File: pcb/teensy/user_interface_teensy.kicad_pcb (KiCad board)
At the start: 2 copper layers, 63.5 x 40.6 mm, 15 parts, among them P1 HEADER_02X08_SMD, SW1 SPST_SLIDE_AS, U1 TLE7230R

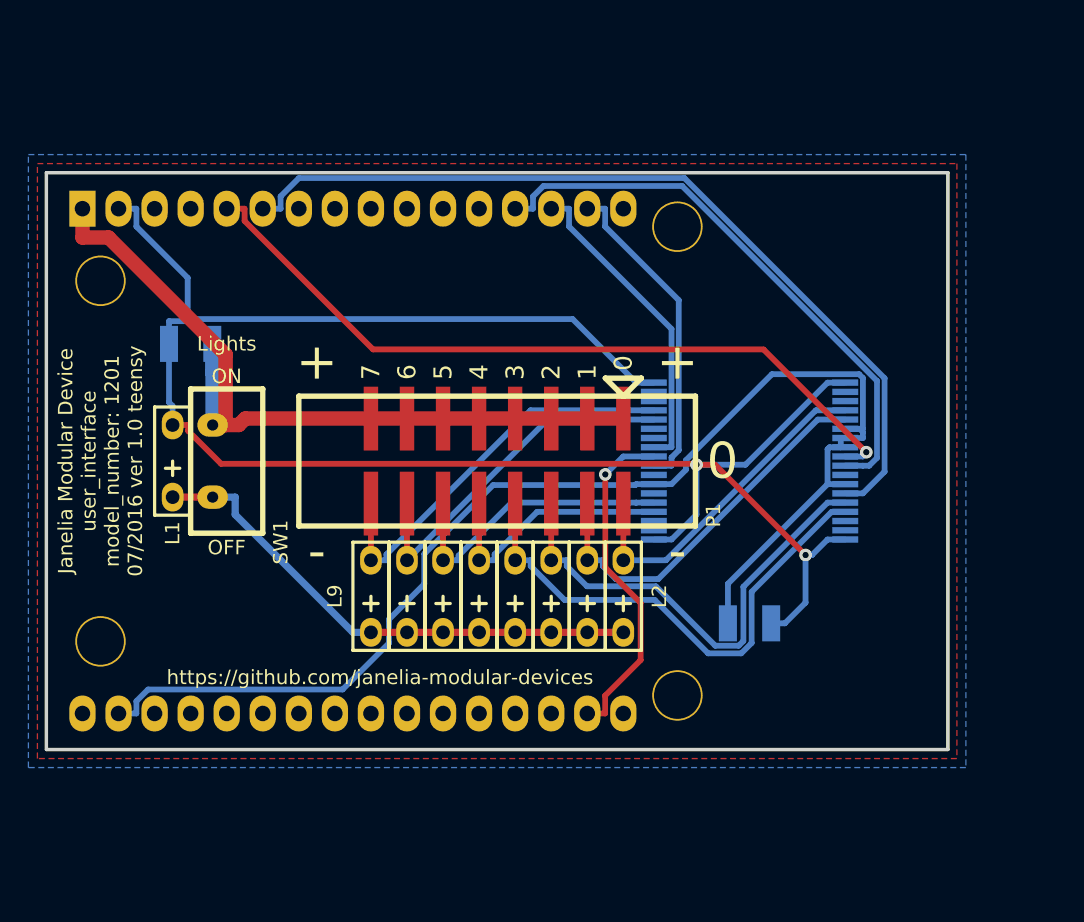
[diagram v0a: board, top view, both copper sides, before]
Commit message: Finished pcb v1.0.
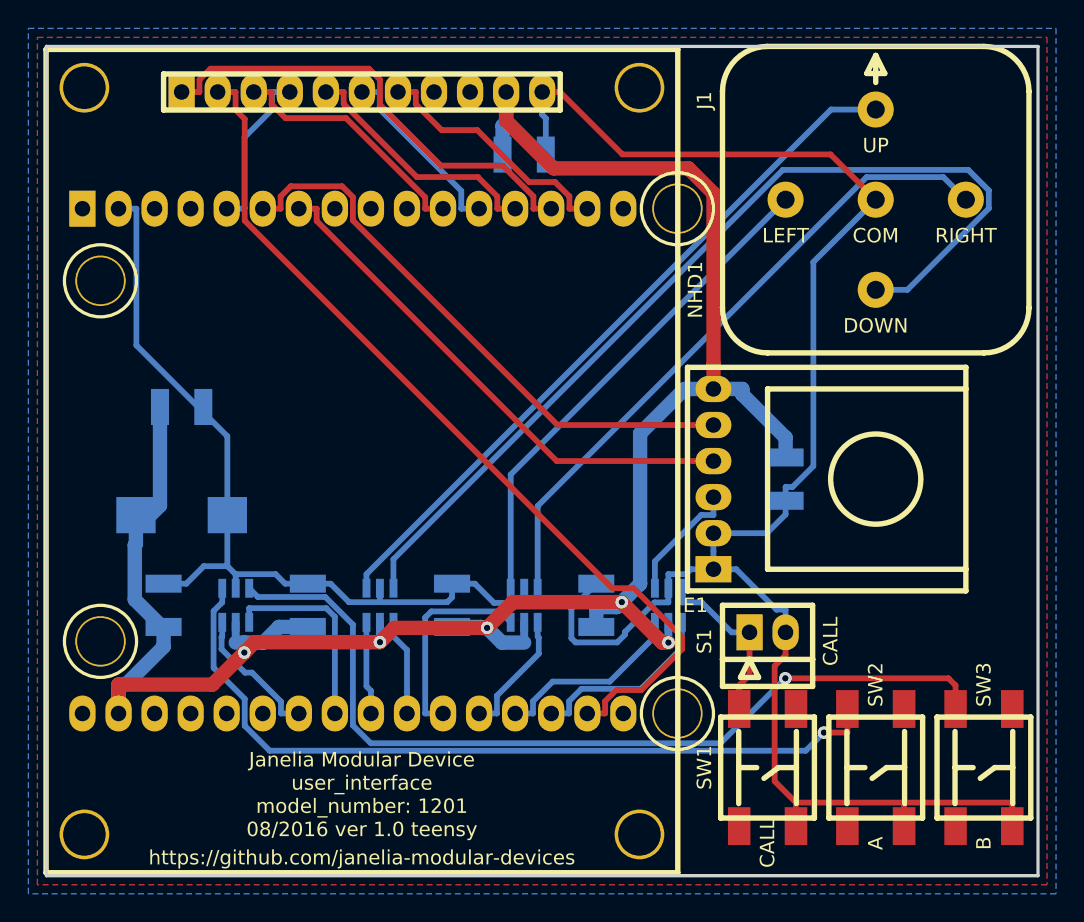
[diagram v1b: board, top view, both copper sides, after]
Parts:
- removed L1, L2, L3, L4, L5, L6, L7, L8, L9: LED_24V, user_interface_teensy:LED_555-3XXX
- removed P1: HEADER_02X08_SMD, user_interface_teensy:HEADER_02x08_SMD
- added C3: 0.1uF, user_interface_teensy:SM1210, B.Cu at (107.3, 78.1)
- added C4: 0.1uF, user_interface_teensy:SM1210, B.Cu at (125.7, 101.0)
- added C5: 0.1uF, user_interface_teensy:SM1210, B.Cu at (112.4, 109.9)
- added C6: 0.1uF, user_interface_teensy:SM1210, B.Cu at (102.2, 109.9)
- added C7: 0.1uF, user_interface_teensy:SM1210, B.Cu at (92.1, 109.9)
- added C8: 0.1uF, user_interface_teensy:SM1210, B.Cu at (81.9, 109.9)
- added E1: ENCODER_62A11-02-P, user_interface_teensy:ENCODER_62AVD, F.Cu at (132.1, 101.0)
- added J1: JOYSTICK, user_interface_teensy:JOYSTICK, F.Cu at (132.1, 81.3)
- added NHD1: NHD-ASC3-169, user_interface_teensy:NHD-ASC3, F.Cu at (95.9, 99.7)
- added S1: HEADER_01X02_SHR, user_interface_teensy:Header_Shrouded_2_Pin, F.Cu at (124.5, 111.8)
- added SW2: KT_SWITCH, user_interface_teensy:KT_SWITCH, F.Cu at (132.1, 121.3)
- added SW3: KT_SWITCH, user_interface_teensy:KT_SWITCH, F.Cu at (139.7, 121.3)
- added U2: MAX6817, user_interface_teensy:MAX6817, B.Cu at (107.3, 109.9)
- added U3: MAX6817, user_interface_teensy:MAX6817, B.Cu at (97.2, 109.9)
- added U4: MAX6817, user_interface_teensy:MAX6817, B.Cu at (87.0, 109.9)
- C2: value 0.1uF -> 10uF; footprint user_interface_teensy:SM1210 -> user_interface_teensy:SM2917_POL
- MDT1: footprint user_interface_teensy:MODULAR_DEVICE_TEENSY -> user_interface_teensy:MODULAR_DEVICE_TEENSY_MALE
- SW1: value SPST_SLIDE_AS -> KT_SWITCH; footprint user_interface_teensy:SPST_SLIDE_AS -> user_interface_teensy:KT_SWITCH
- U1: value TLE7230R -> MAX6817; footprint user_interface_teensy:PG-DSO-36 -> user_interface_teensy:MAX6817
- moved SW1 43.8 mm to (124.5, 121.3), turned to 90 degrees
- moved C2 40.7 mm to (83.2, 103.5)
- moved U1 11.7 mm to (117.5, 109.9)
- moved C1 4.49 mm to (83.2, 95.9), turned to 0 degrees
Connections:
- C1 pad 1: VDD -> VEE
- MDT1 pad 10: /CS -> /OLEDCS
- MDT1 pad 14: (no net) -> /BTN_CALL
- MDT1 pad 15: (no net) -> /BTN_ENC
- MDT1 pad 16: (no net) -> /RIGHT
- MDT1 pad 17: (no net) -> /LEFT
- MDT1 pad 18: (no net) -> /DOWN
- MDT1 pad 19: (no net) -> /UP
- MDT1 pad 20: (no net) -> /BTN_B
- MDT1 pad 21: (no net) -> /BTN_A
- MDT1 pad 29: (no net) -> /OLEDDC
- MDT1 pad 3: /PWM -> /ENC_A
- MDT1 pad 4: (no net) -> /ENC_B
- MDT1 pad 9: (no net) -> /SDCS
- MDT1 pad VDD: VDD -> (no net)
- SW1 pad 1: VDD -> (no net)
- SW1 pad 3: /LED_PWR -> GND
- U1 pad 1: GND -> /B_BTN_ENC
- U1 pad 2: (no net) -> GND
- U1 pad 3: (no net) -> /B_BTN_CALL
- U1 pad 4: /OUT0 -> /BTN_CALL
- U1 pad 5: /OUT1 -> VEE
- U1 pad 6: VEE -> /BTN_ENC
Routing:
- net /B_DOWN: track 0.00 -> 67.6 mm
- net VEE: track 91.1 -> 155.1 mm, vias 0 -> 5
- net /B_BTN_B: track 0.00 -> 62.2 mm, vias 0 -> 1
- net /PWM: track 61.0 -> 0.00 mm
- net /B_BTN_A: track 0.00 -> 56.2 mm, vias 0 -> 1
- net GND: track 132.4 -> 188.0 mm, vias 2 -> 0
- net VDD: track 55.3 -> 0.00 mm
- net /B_UP: track 0.00 -> 50.4 mm
- net /B_RIGHT: track 0.00 -> 46.2 mm
- net /RESET: track 54.3 -> 11.5 mm, vias 1 -> 0
- net /ENC_A: track 0.00 -> 40.8 mm
- net /CS: track 40.2 -> 0.00 mm
- net /SCK: track 24.1 -> 63.5 mm, vias 1 -> 0
- net /ENC_B: track 0.00 -> 37.1 mm
- net /OUT3: track 36.4 -> 0.00 mm
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- added copper zone on F.Cu, net VEE
- removed copper zone on F.Cu, net VDD
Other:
- board size 63.5 x 40.6 mm -> 69.8 x 58.4 mm
- board text added: "CALL"
- board text added: "Janelia Modular Device user_interface model_number: 1201 08/2016 ver 1.0 teensy"
- board text removed: "+"
- board text removed: "-"
- board text removed: "0"
- board text removed: "1"
- board text removed: "2"
- board text removed: "3"
- board text removed: "4"
- board text removed: "5"
- board text removed: "6"
- board text removed: "7"
- board text removed: "Janelia Modular Device user_interface model_number: 1201 07/2016 ver 1.0 teensy"
- board text removed: "Lights"
